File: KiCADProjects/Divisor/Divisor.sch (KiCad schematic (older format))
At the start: 34 parts, among them J1 SMA_Female, J10 SMA_Female, J11 SMA_Female, J12 SMA_Female, J13 SMA_Female, J14 SMA_Female, J15 SMA_Female, J16 SMA_Female, J17 SMA_Female, J2 SMA_Female, J3 SMA_Female, J4 SMA_Female, J5 SMA_Female, J6 SMA_Female, J7 SMA_Female, J8 SMA_Female, J9 SMA_Female

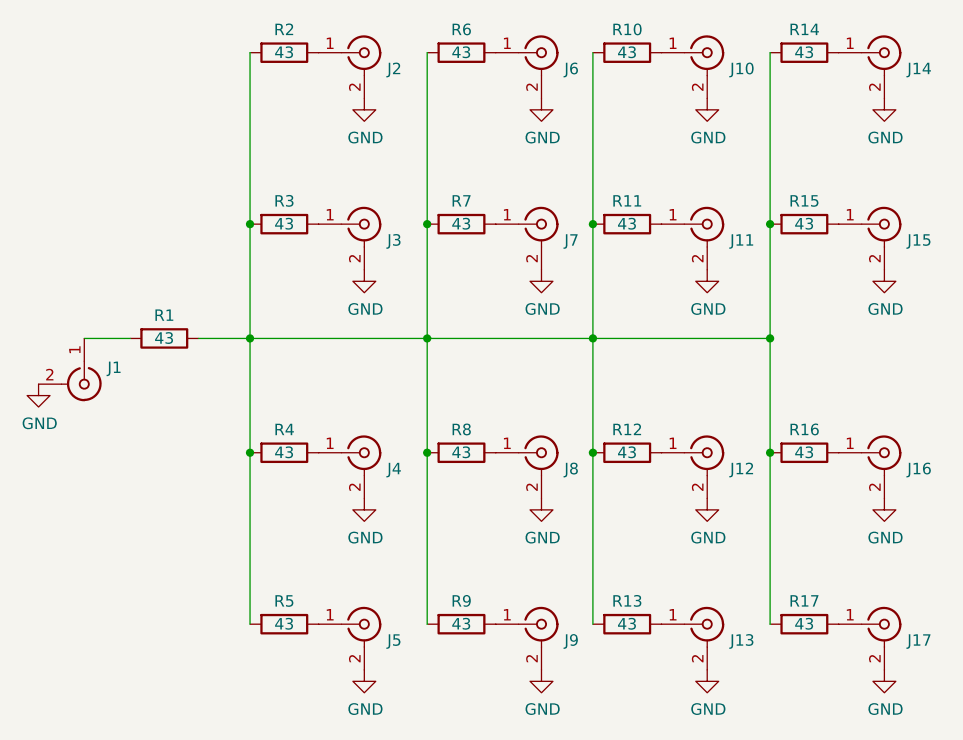
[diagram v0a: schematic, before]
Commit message: Revisión 1.1 de PCBs
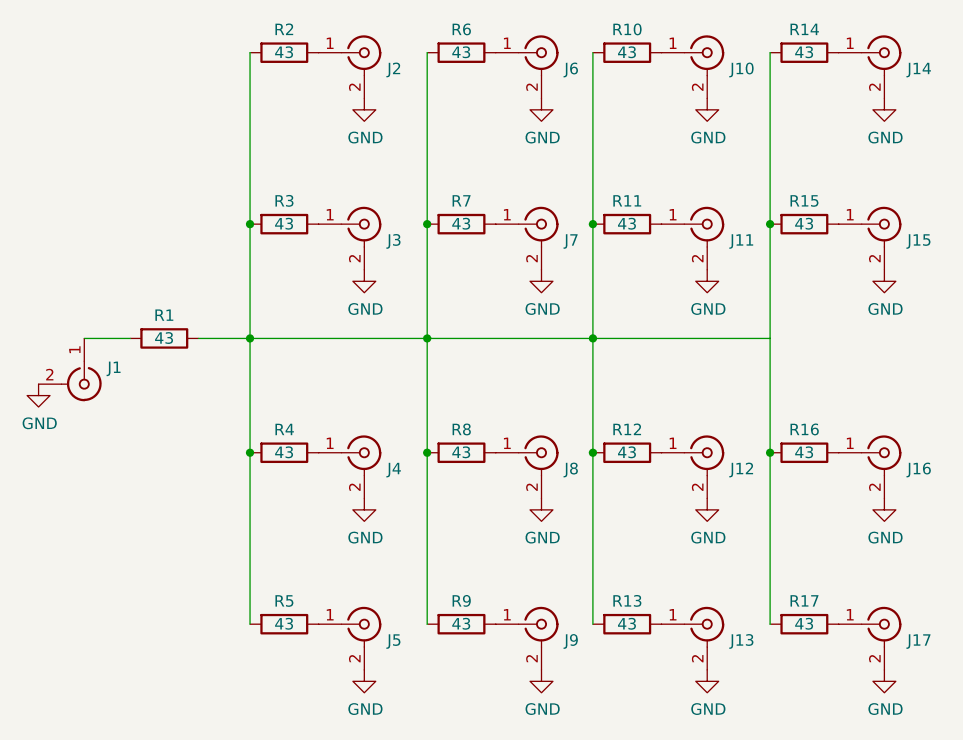
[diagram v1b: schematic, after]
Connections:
- wire segments 21 -> 20
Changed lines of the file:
@@
 	6250 4150 6250 4900
 Connection ~ 7025 3150
-Wire Wire Line
-	7025 3150 7025 3650
-Connection ~ 7025 3650
-Wire Wire Line
-	7025 3650 7025 4150
 Connection ~ 7025 4150
 Wire Wire Line
@@
 	1    0    0    -1
 $EndComp
+Wire Wire Line
+	7025 3150 7025 4150
 $EndSCHEMATC
